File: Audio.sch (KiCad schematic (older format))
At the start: 53 parts, among them J5 PJ-3270, J6 PJ-3270, J7 PJ-3270, U6 SSM2603, Y1 12.288Mhz

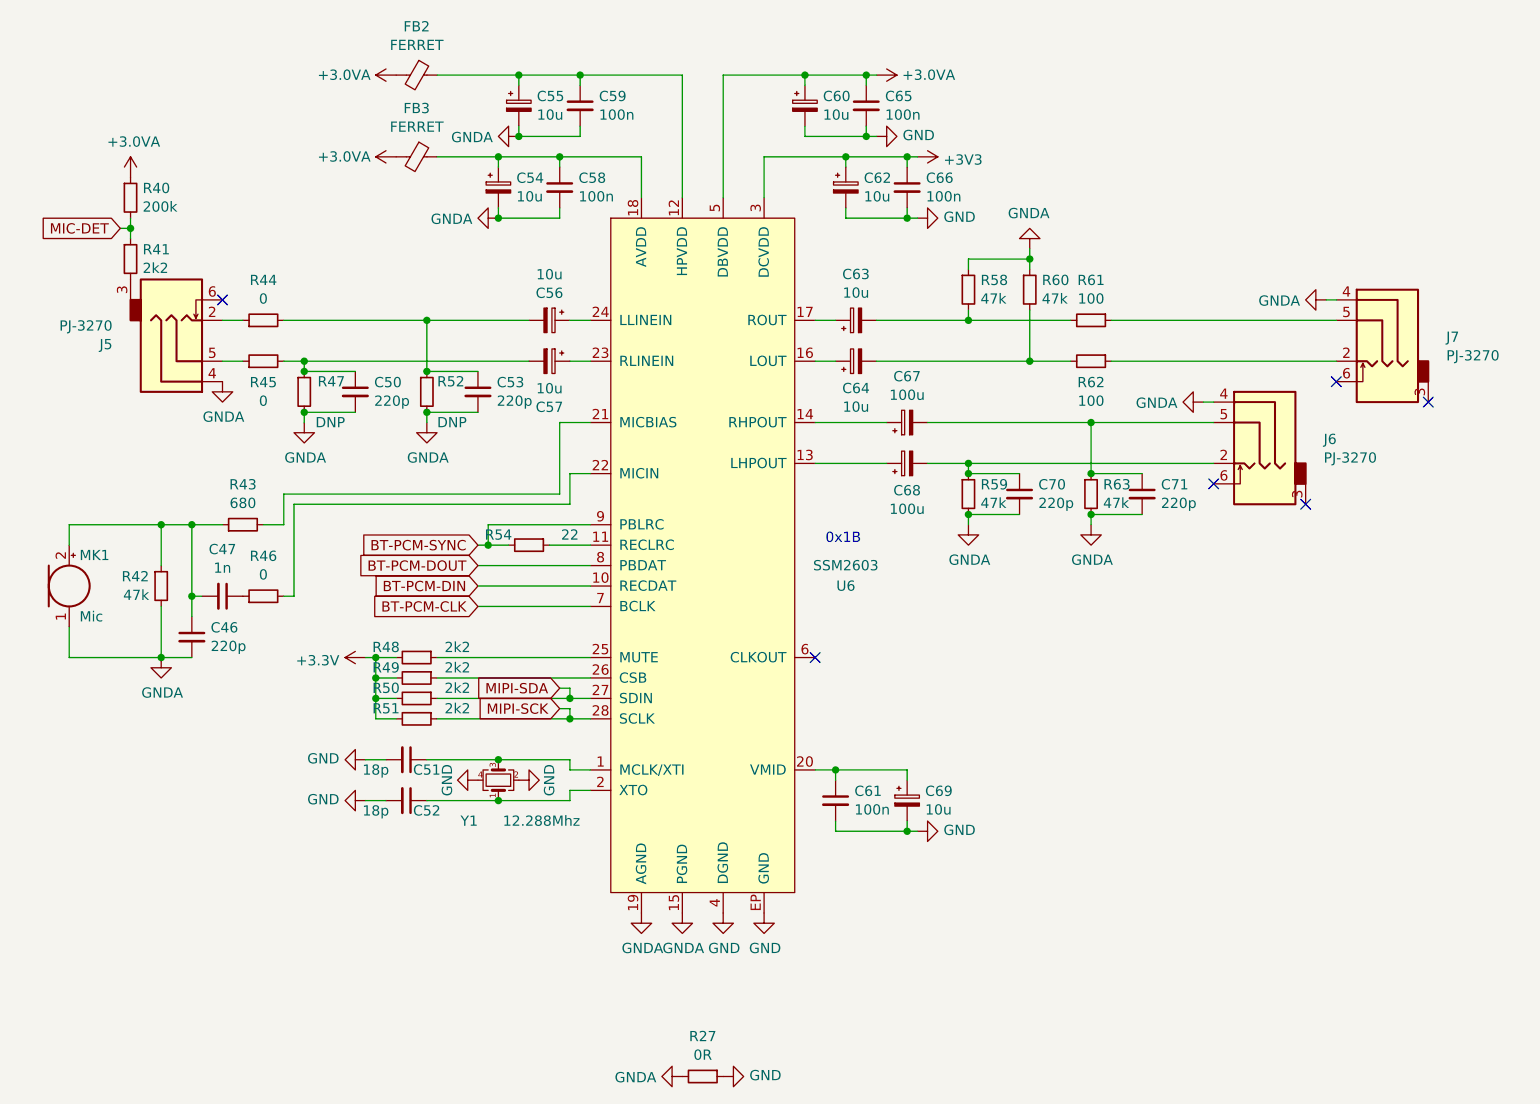
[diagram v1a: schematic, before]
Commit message: beautify kicad project
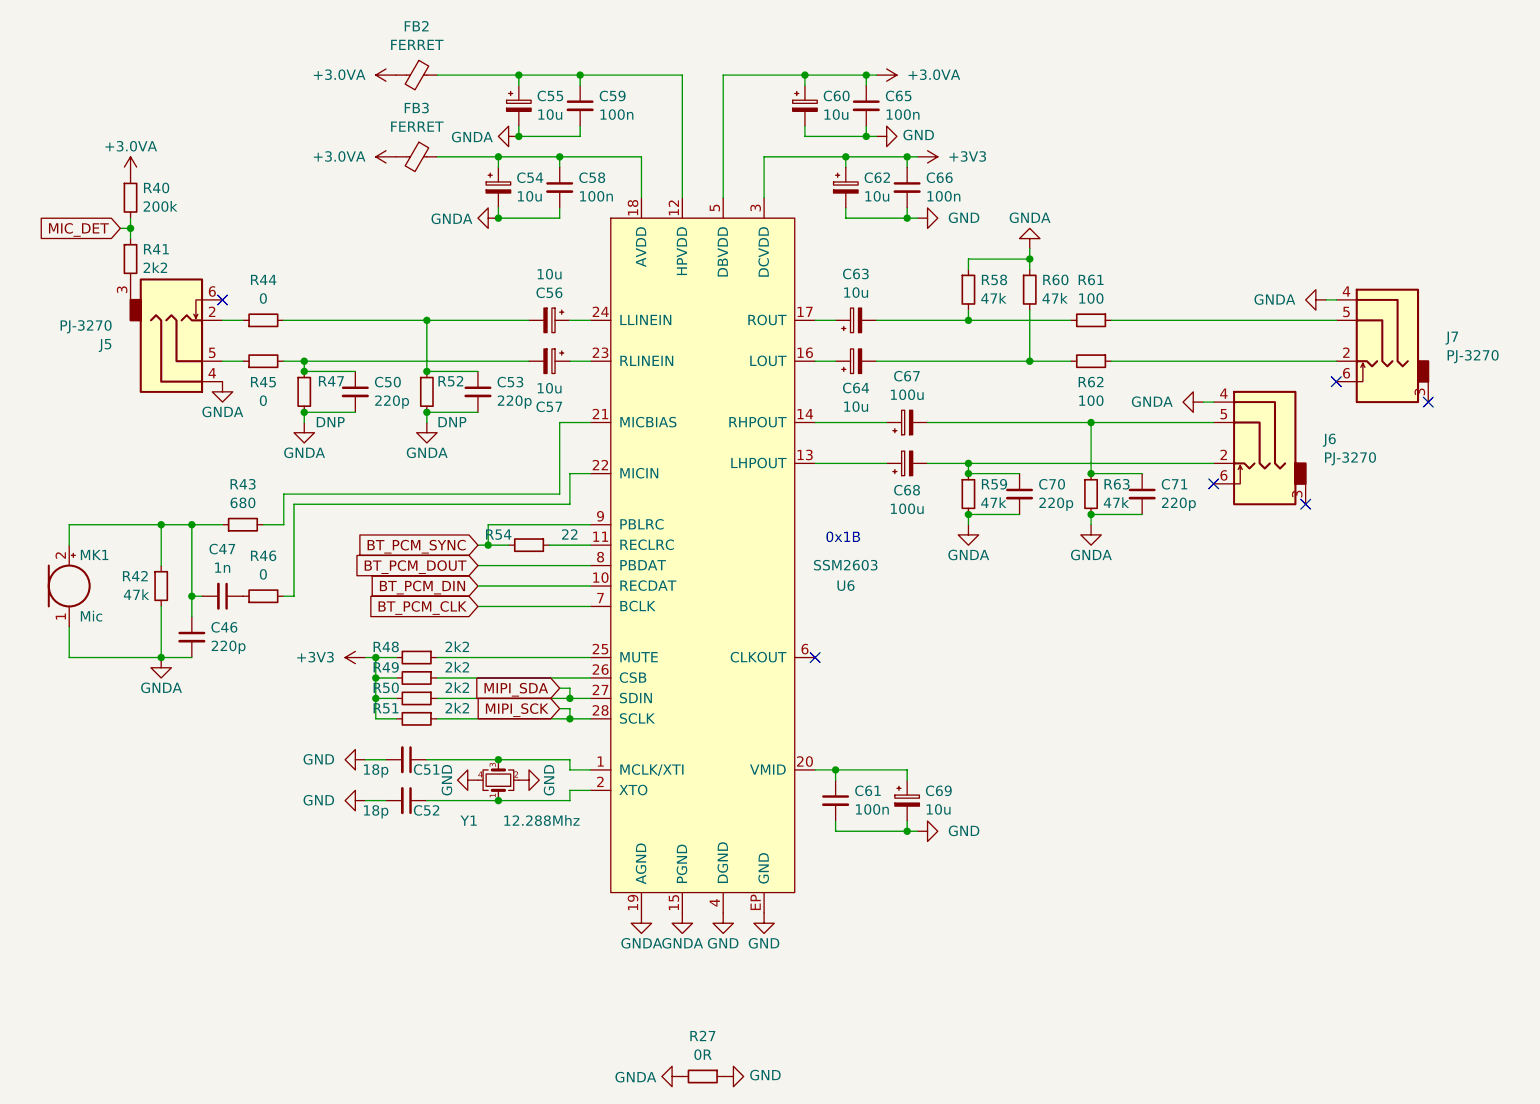
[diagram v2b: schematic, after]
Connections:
- net BT-PCM-CLK renamed BT_PCM_CLK
- net BT-PCM-DIN renamed BT_PCM_DIN
- net BT-PCM-DOUT renamed BT_PCM_DOUT
- net BT-PCM-SYNC renamed BT_PCM_SYNC
- net MIC-DET renamed MIC_DET
- net MIPI-SCK renamed MIPI_SCK
- net MIPI-SDA renamed MIPI_SDA
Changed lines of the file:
@@
 $EndDescr
 Text GLabel 4650 4000 0    50   Input ~ 0
-BT-PCM-SYNC
+BT_PCM_SYNC
 Text GLabel 4650 4300 0    50   Input ~ 0
-BT-PCM-CLK
+BT_PCM_CLK
 Text GLabel 4650 4200 0    50   Input ~ 0
-BT-PCM-DIN
+BT_PCM_DIN
 Text GLabel 4650 4100 0    50   Input ~ 0
-BT-PCM-DOUT
+BT_PCM_DOUT
 $Comp
 L otter:SSM2603 U6
@@
 P 5850 5800
 F 0 "#PWR0205" H 5850 5550 50  0001 C CNN
-F 1 "GND" H 5855 5627 50  0000 C CNN
+F 1 "GND" H 5850 5650 50  0000 C CNN
 F 2 "" H 5850 5800 60  0000 C CNN
 F 3 "" H 5850 5800 60  0000 C CNN
@@
 P 6050 5800
 F 0 "#PWR0206" H 6050 5550 50  0001 C CNN
-F 1 "GND" H 6055 5627 50  0000 C CNN
+F 1 "GND" H 6050 5650 50  0000 C CNN
 F 2 "" H 6050 5800 60  0000 C CNN
 F 3 "" H 6050 5800 60  0000 C CNN
@@
 $EndComp
 $Comp
-L OtterCastAudioV2-rescue:GND-S3-OLinuXino_Rev_A #PWR?
+L power:GND #PWR?
 U 1 1 5FF96B43
 P 4850 5150
@@
 Connection ~ 4750 5250
 $Comp
-L OtterCastAudioV2-rescue:GND-S3-OLinuXino_Rev_A #PWR?
+L power:GND #PWR?
 U 1 1 5FF96B59
 P 4650 5150
@@
 	4750 5250 4400 5250
 $Comp
-L OtterCastAudioV2-rescue:GND-S3-OLinuXino_Rev_A #PWR?
+L power:GND #PWR?
 U 1 1 5FF96B61
 P 4100 5050
@@
 AR Path="/604A1CEE/5FF96B61" Ref="#PWR0209"  Part="1"
 F 0 "#PWR0209" H 4100 4800 50  0001 C CNN
-F 1 "GND" V 4105 4922 50  0000 R CNN
+F 1 "GND" V 4100 4900 50  0000 R CNN
 F 2 "" H 4100 5050 60  0000 C CNN
 F 3 "" H 4100 5050 60  0000 C CNN
@@
 	4100 5050 4200 5050
 $Comp
-L OtterCastAudioV2-rescue:GND-S3-OLinuXino_Rev_A #PWR?
+L power:GND #PWR?
 U 1 1 5FF96B68
 P 4100 5250
@@
 AR Path="/604A1CEE/5FF96B68" Ref="#PWR0210"  Part="1"
 F 0 "#PWR0210" H 4100 5000 50  0001 C CNN
-F 1 "GND" V 4105 5122 50  0000 R CNN
+F 1 "GND" V 4100 5100 50  0000 R CNN
 F 2 "" H 4100 5250 60  0000 C CNN
 F 3 "" H 4100 5250 60  0000 C CNN
@@
 	0    1    1    0
 $EndComp
-$Comp
-L OtterCastAudioV2-rescue:+3.3V-S3-OLinuXino_Rev_A #PWR?
-U 1 1 5FFB96F5
-P 4100 4550
-AR Path="/5D8A1FAC/5FFB96F5" Ref="#PWR?"  Part="1"
-AR Path="/5FFB96F5" Ref="#PWR?"  Part="1"
-AR Path="/602ACDF9/5FFB96F5" Ref="#PWR?"  Part="1"
-AR Path="/604A1CEE/5FFB96F5" Ref="#PWR0211"  Part="1"
-F 0 "#PWR0211" H 4100 4400 50  0001 C CNN
-F 1 "+3.3V" V 4115 4678 50  0000 L CNN
-F 2 "" H 4100 4550 60  0000 C CNN
-F 3 "" H 4100 4550 60  0000 C CNN
-	1    4100 4550
-	0    -1   1    0
-$EndComp
 Wire Wire Line
 	4250 4750 4150 4750
@@
 Wire Wire Line
 	4750 2400 4750 2350
-$Comp
-L power:+3V3 #PWR0212
-U 1 1 601B1CBC
-P 6800 2100
-F 0 "#PWR0212" H 6800 1950 50  0001 C CNN
-F 1 "+3V3" V 6815 2228 50  0000 L CNN
-F 2 "" H 6800 2100 50  0001 C CNN
-F 3 "" H 6800 2100 50  0001 C CNN
-	1    6800 2100
-	0    1    1    0
-$EndComp
 Wire Wire Line
 	6800 2100 6750 2100
@@
 P 6800 2400
 F 0 "#PWR0213" H 6800 2150 50  0001 C CNN
-F 1 "GND" V 6805 2272 50  0000 R CNN
+F 1 "GND" V 6800 2250 50  0000 R CNN
 F 2 "" H 6800 2400 60  0000 C CNN
 F 3 "" H 6800 2400 60  0000 C CNN
@@
 Wire Wire Line
 	4850 1700 5150 1700
-$Comp
-L OtterCastAudioV2-rescue:+3.0VA-S3-OLinuXino_Rev_A #PWR?
-U 1 1 6023A1C9
-P 6600 1700
-AR Path="/5D8A1FAC/6023A1C9" Ref="#PWR?"  Part="1"
-AR Path="/6023A1C9" Ref="#PWR?"  Part="1"
-AR Path="/602ACDF9/6023A1C9" Ref="#PWR?"  Part="1"
-AR Path="/604A1CEE/6023A1C9" Ref="#PWR0215"  Part="1"
-F 0 "#PWR0215" H 6600 1550 50  0001 C CNN
-F 1 "+3.0VA" V 6600 1825 50  0000 L CNN
-F 2 "" H 6600 1700 60  0000 C CNN
-F 3 "" H 6600 1700 60  0000 C CNN
-	1    6600 1700
-	0    1    1    0
-$EndComp
 Wire Wire Line
 	6600 1700 6550 1700
@@
 Connection ~ 4850 1700
 $Comp
-L OtterCastAudioV2-rescue:+3.0VA-S3-OLinuXino_Rev_A #PWR?
-U 1 1 6027AD71
-P 4250 1700
-AR Path="/5D8A1FAC/6027AD71" Ref="#PWR?"  Part="1"
-AR Path="/6027AD71" Ref="#PWR?"  Part="1"
-AR Path="/602ACDF9/6027AD71" Ref="#PWR?"  Part="1"
-AR Path="/604A1CEE/6027AD71" Ref="#PWR0216"  Part="1"
-F 0 "#PWR0216" H 4250 1550 50  0001 C CNN
-F 1 "+3.0VA" V 4250 1825 50  0000 L CNN
-F 2 "" H 4250 1700 60  0000 C CNN
-F 3 "" H 4250 1700 60  0000 C CNN
-	1    4250 1700
-	0    -1   -1   0
-$EndComp
-$Comp
 L power:GNDA #PWR0217
 U 1 1 6029A1CD
@@
 	1    4750 2400
 	0    1    1    0
-$EndComp
-$Comp
-L OtterCastAudioV2-rescue:+3.0VA-S3-OLinuXino_Rev_A #PWR?
-U 1 1 602F2215
-P 4250 2100
-AR Path="/5D8A1FAC/602F2215" Ref="#PWR?"  Part="1"
-AR Path="/602F2215" Ref="#PWR?"  Part="1"
-AR Path="/602ACDF9/602F2215" Ref="#PWR?"  Part="1"
-AR Path="/604A1CEE/602F2215" Ref="#PWR0220"  Part="1"
-F 0 "#PWR0220" H 4250 1950 50  0001 C CNN
-F 1 "+3.0VA" V 4250 2225 50  0000 L CNN
-F 2 "" H 4250 2100 60  0000 C CNN
-F 3 "" H 4250 2100 60  0000 C CNN
-	1    4250 2100
-	0    -1   -1   0
 $EndComp
 $Comp
@@
 P 7350 2550
 F 0 "#PWR0222" H 7350 2300 50  0001 C CNN
-F 1 "GNDA" H 7355 2377 50  0000 C CNN
+F 1 "GNDA" H 7350 2400 50  0000 C CNN
 F 2 "" H 7350 2550 50  0001 C CNN
 F 3 "" H 7350 2550 50  0001 C CNN
@@
 P 8800 2800
 F 0 "#PWR0223" H 8800 2550 50  0001 C CNN
-F 1 "GNDA" V 8805 2673 50  0000 R CNN
+F 1 "GNDA" V 8800 2650 50  0000 R CNN
 F 2 "" H 8800 2800 50  0001 C CNN
 F 3 "" H 8800 2800 50  0001 C CNN
@@
 P 7050 3900
 F 0 "#PWR0224" H 7050 3650 50  0001 C CNN
-F 1 "GNDA" H 7055 3727 50  0000 C CNN
+F 1 "GNDA" H 7050 3750 50  0000 C CNN
 F 2 "" H 7050 3900 50  0001 C CNN
 F 3 "" H 7050 3900 50  0001 C CNN
@@
 P 7650 3900
 F 0 "#PWR0225" H 7650 3650 50  0001 C CNN
-F 1 "GNDA" H 7655 3727 50  0000 C CNN
+F 1 "GNDA" H 7650 3750 50  0000 C CNN
 F 2 "" H 7650 3900 50  0001 C CNN
 F 3 "" H 7650 3900 50  0001 C CNN
@@
 P 8200 3300
 F 0 "#PWR0226" H 8200 3050 50  0001 C CNN
-F 1 "GNDA" V 8205 3173 50  0000 R CNN
+F 1 "GNDA" V 8200 3150 50  0000 R CNN
 F 2 "" H 8200 3300 50  0001 C CNN
 F 3 "" H 8200 3300 50  0001 C CNN
@@
 P 3800 3400
 F 0 "#PWR0227" H 3800 3150 50  0001 C CNN
-F 1 "GNDA" H 3805 3227 50  0000 C CNN
+F 1 "GNDA" H 3800 3250 50  0000 C CNN
 F 2 "" H 3800 3400 50  0001 C CNN
 F 3 "" H 3800 3400 50  0001 C CNN
@@
 P 4400 3400
 F 0 "#PWR0228" H 4400 3150 50  0001 C CNN
-F 1 "GNDA" H 4405 3227 50  0000 C CNN
+F 1 "GNDA" H 4400 3250 50  0000 C CNN
 F 2 "" H 4400 3400 50  0001 C CNN
 F 3 "" H 4400 3400 50  0001 C CNN
@@
 P 3400 3200
 F 0 "#PWR0229" H 3400 2950 50  0001 C CNN
-F 1 "GNDA" H 3405 3027 50  0000 C CNN
+F 1 "GNDA" H 3400 3050 50  0000 C CNN
 F 2 "" H 3400 3200 50  0001 C CNN
 F 3 "" H 3400 3200 50  0001 C CNN
@@
 P 3100 4550
 F 0 "#PWR0230" H 3100 4300 50  0001 C CNN
-F 1 "GNDA" H 3105 4377 50  0000 C CNN
+F 1 "GNDA" H 3100 4400 50  0000 C CNN
 F 2 "" H 3100 4550 50  0001 C CNN
 F 3 "" H 3100 4550 50  0001 C CNN
@@
 P 6800 5400
 F 0 "#PWR0231" H 6800 5150 50  0001 C CNN
-F 1 "GND" V 6805 5272 50  0000 R CNN
+F 1 "GND" V 6800 5250 50  0000 R CNN
 F 2 "" H 6800 5400 60  0000 C CNN
 F 3 "" H 6800 5400 60  0000 C CNN
@@
 Wire Wire Line
 	2950 2500 2950 2450
-$Comp
-L OtterCastAudioV2-rescue:+3.0VA-S3-OLinuXino_Rev_A #PWR?
-U 1 1 60C3B44B
-P 2950 2200
-AR Path="/5D8A1FAC/60C3B44B" Ref="#PWR?"  Part="1"
-AR Path="/60C3B44B" Ref="#PWR?"  Part="1"
-AR Path="/602ACDF9/60C3B44B" Ref="#PWR?"  Part="1"
-AR Path="/604A1CEE/60C3B44B" Ref="#PWR0232"  Part="1"
-F 0 "#PWR0232" H 2950 2050 50  0001 C CNN
-F 1 "+3.0VA" H 2965 2373 50  0000 C CNN
-F 2 "" H 2950 2200 60  0000 C CNN
-F 3 "" H 2950 2200 60  0000 C CNN
-	1    2950 2200
-	1    0    0    -1
-$EndComp
 Text GLabel 2900 2450 0    50   Input ~ 0
-MIC-DET
+MIC_DET
 NoConn ~ 9300 3300
 NoConn ~ 8700 3800
@@
 P 5650 5800
 F 0 "#PWR0155" H 5650 5550 50  0001 C CNN
-F 1 "GNDA" H 5655 5627 50  0000 C CNN
+F 1 "GNDA" H 5650 5650 50  0000 C CNN
 F 2 "" H 5650 5800 50  0001 C CNN
 F 3 "" H 5650 5800 50  0001 C CNN
@@
 P 5450 5800
 F 0 "#PWR0203" H 5450 5550 50  0001 C CNN
-F 1 "GNDA" H 5455 5627 50  0000 C CNN
+F 1 "GNDA" H 5450 5650 50  0000 C CNN
 F 2 "" H 5450 5800 50  0001 C CNN
 F 3 "" H 5450 5800 50  0001 C CNN
@@
 $EndComp
 Text GLabel 5050 4700 0    50   Input ~ 0
-MIPI-SDA
+MIPI_SDA
 Text GLabel 5050 4800 0    50   Input ~ 0
-MIPI-SCK
+MIPI_SCK
 Wire Wire Line
 	5050 4800 5100 4800
@@
 	0    1    1    0
 $EndComp
+$Comp
+L power:+3V3 #PWR?
+U 1 1 604083EC
+P 6800 2100
+F 0 "#PWR?" H 6800 1950 50  0001 C CNN
+F 1 "+3V3" V 6800 2250 50  0000 L CNN
+F 2 "" H 6800 2100 50  0001 C CNN
+F 3 "" H 6800 2100 50  0001 C CNN
+	1    6800 2100
+	0    1    1    0
+$EndComp
+$Comp
+L power:+3V3 #PWR?
+U 1 1 604097B1
+P 4100 4550
+F 0 "#PWR?" H 4100 4400 50  0001 C CNN
+F 1 "+3V3" V 4100 4700 50  0000 L CNN
+F 2 "" H 4100 4550 50  0001 C CNN
+F 3 "" H 4100 4550 50  0001 C CNN
+	1    4100 4550
+	0    -1   -1   0
+$EndComp
+$Comp
+L otter:+3.0VA #PWR?
+U 1 1 606F1C66
+P 6600 1700
+AR Path="/602ACDF9/606F1C66" Ref="#PWR?"  Part="1"
+AR Path="/604A1CEE/606F1C66" Ref="#PWR?"  Part="1"
+F 0 "#PWR?" H 6600 1550 50  0001 C CNN
+F 1 "+3.0VA" V 6600 1850 50  0000 L CNN
+F 2 "" H 6600 1700 60  0000 C CNN
+F 3 "" H 6600 1700 60  0000 C CNN
+	1    6600 1700
+	0    1    1    0
+$EndComp
+$Comp
+L otter:+3.0VA #PWR?
+U 1 1 606F8C84
+P 4250 1700
+AR Path="/602ACDF9/606F8C84" Ref="#PWR?"  Part="1"
+AR Path="/604A1CEE/606F8C84" Ref="#PWR?"  Part="1"
+F 0 "#PWR?" H 4250 1550 50  0001 C CNN
+F 1 "+3.0VA" V 4250 1850 50  0000 L CNN
+F 2 "" H 4250 1700 60  0000 C CNN
+F 3 "" H 4250 1700 60  0000 C CNN
+	1    4250 1700
+	0    -1   -1   0
+$EndComp
+$Comp
+L otter:+3.0VA #PWR?
+U 1 1 606FFCD1
+P 4250 2100
+AR Path="/602ACDF9/606FFCD1" Ref="#PWR?"  Part="1"
+AR Path="/604A1CEE/606FFCD1" Ref="#PWR?"  Part="1"
+F 0 "#PWR?" H 4250 1950 50  0001 C CNN
+F 1 "+3.0VA" V 4250 2250 50  0000 L CNN
+F 2 "" H 4250 2100 60  0000 C CNN
+F 3 "" H 4250 2100 60  0000 C CNN
+	1    4250 2100
+	0    -1   -1   0
+$EndComp
+$Comp
+L otter:+3.0VA #PWR?
+U 1 1 60706D98
+P 2950 2200
+AR Path="/602ACDF9/60706D98" Ref="#PWR?"  Part="1"
+AR Path="/604A1CEE/60706D98" Ref="#PWR?"  Part="1"
+F 0 "#PWR?" H 2950 2050 50  0001 C CNN
+F 1 "+3.0VA" H 2950 2350 50  0000 C CNN
+F 2 "" H 2950 2200 60  0000 C CNN
+F 3 "" H 2950 2200 60  0000 C CNN
+	1    2950 2200
+	1    0    0    -1
+$EndComp
 $EndSCHEMATC
